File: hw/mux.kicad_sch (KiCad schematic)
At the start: 6 parts, among them Q1 NMOS, U11 NCP708, U6 TS3USB3031

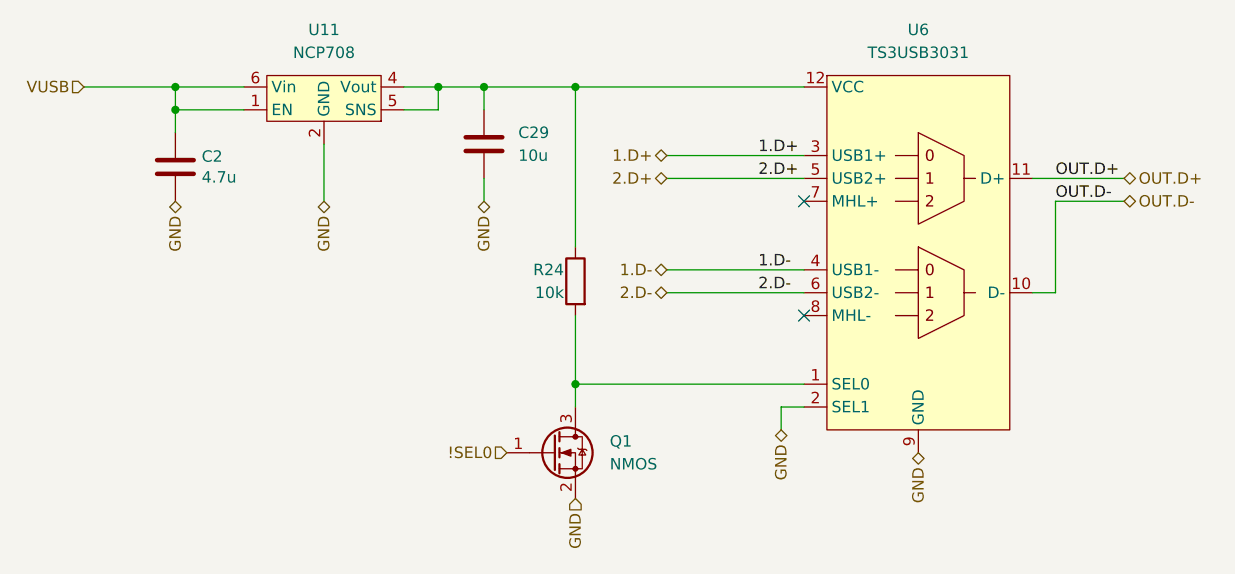
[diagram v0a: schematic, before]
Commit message: a mixture of everything
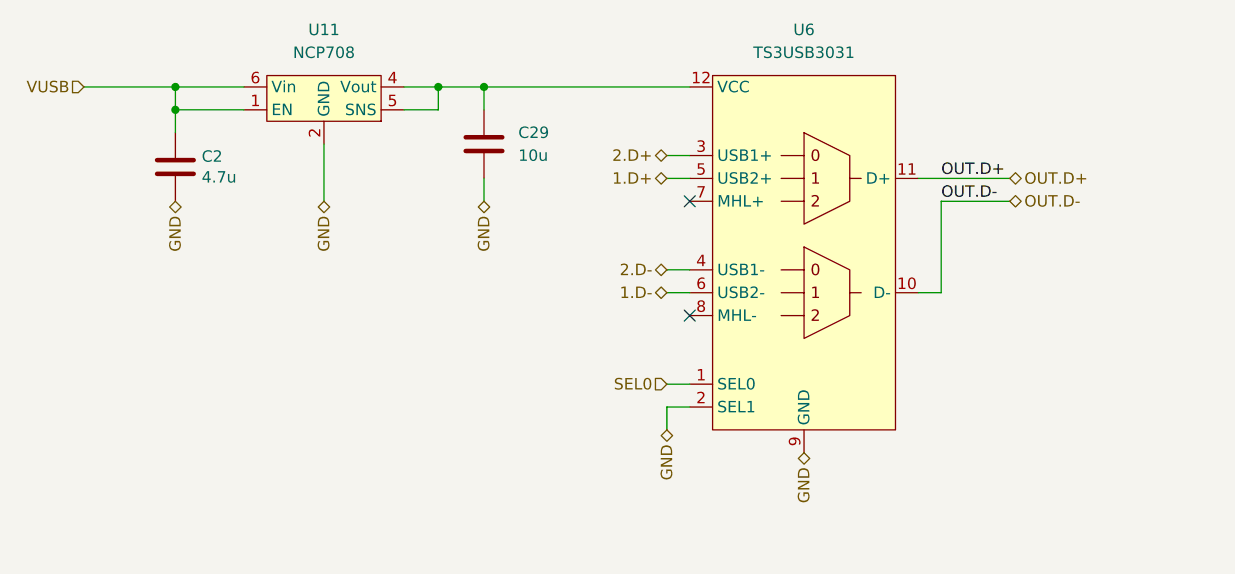
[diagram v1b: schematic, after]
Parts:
- removed Q1: NMOS, Package_TO_SOT_SMD:SOT-723, symbol Device:Q_NMOS_GSD
- removed R24: 10k, Resistor_SMD:R_0402_1005Metric, symbol Device:R
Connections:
- net 1.D+: now also U6.5 (USB2+); no longer U6.3 (USB1+)
- net 1.D-: now also U6.6 (USB2-); no longer U6.4 (USB1-)
- net 2.D+: now also U6.3 (USB1+); no longer U6.5 (USB2+)
- net 2.D-: now also U6.4 (USB1-); no longer U6.6 (USB2-)
- net SEL0: now reaches U6.1 (SEL0)
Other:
- moved on the sheet: U6
